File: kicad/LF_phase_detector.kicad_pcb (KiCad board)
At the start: 2 copper layers, 108 x 99.8 mm, 233 parts, among them M1 NUCLEO-H743ZI, P1 MSTBA 2,5/ 2-G-5,08 - 1757242, T1 AO4485, U1 HMC984LP4E, U10 TMUX1204DGSR, U11 TMUX1204DGSR, U12 TMUX1204DGSR, U13 TMUX1204DGSR, U14 OPA2325, U15 ADA4807-2ARM, U16 ADA4807-2ARM, U17 AP63200WU, U18 AP63203WU-7, U19 L78M05ACDT, U2 TMUX1204DGSR, U20 AP2210N-3.0TRG1, U21 AP2210N-3.0TRG1, U22 AP2210N-5.0TRG1, U23 AP2210N-5.0TRG1, U24 AP2210N-5.0TRG1, U25 GALI-39+, U26 GALI-39+, U27 AD9515BCPZ, U28 AD9515BCPZ, U29 AP2210N-5.0TRG1, U3 TMUX1204DGSR, U4 TMUX1204DGSR, U5 TMUX1204DGSR, U6 TMUX1204DGSR, U7 TMUX1204DGSR, U8 TMUX1204DGSR, U9 TMUX1204DGSR

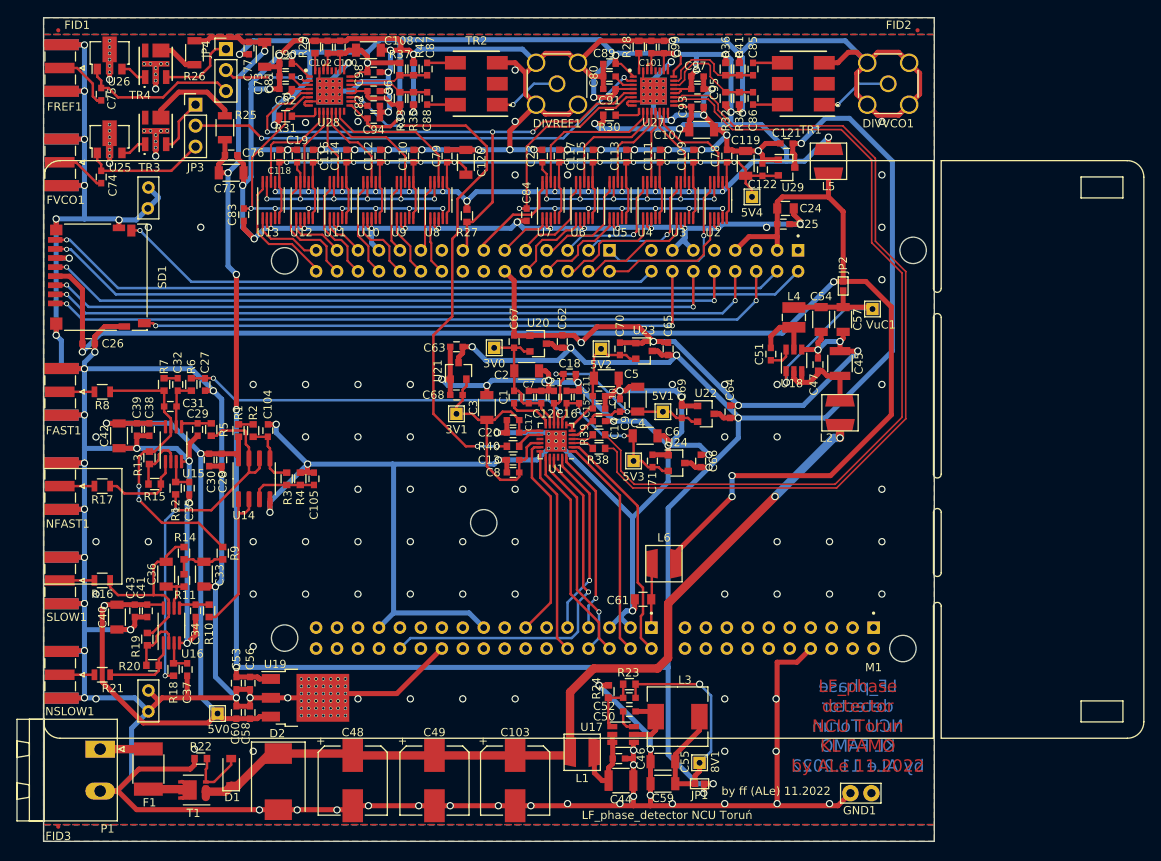
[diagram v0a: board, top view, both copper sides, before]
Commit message: some initial commits
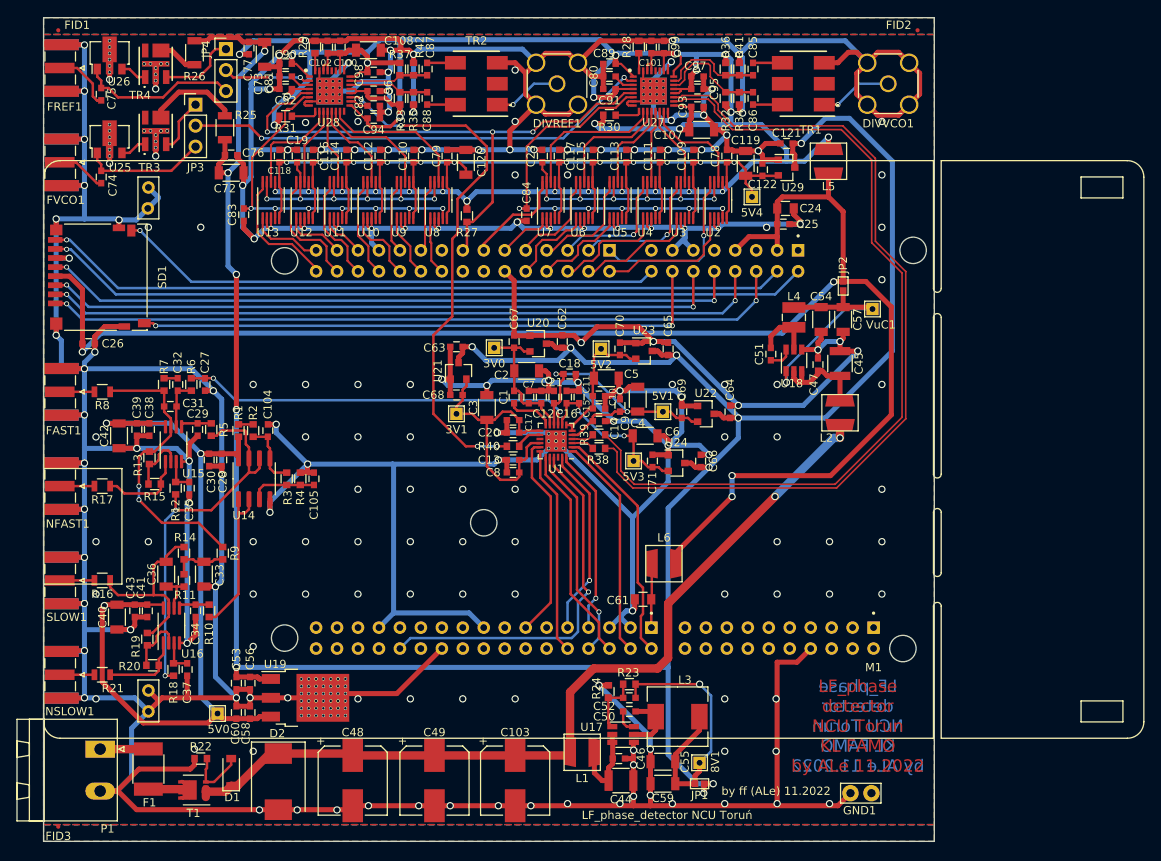
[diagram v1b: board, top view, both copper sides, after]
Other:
- net class 24V removed
- net class Default removed
- net class motor removed
- net class motorii removed
- net class zasilanie 5v removed
